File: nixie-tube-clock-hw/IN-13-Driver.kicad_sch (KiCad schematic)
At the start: 7 parts, among them Q50 FZT857TA

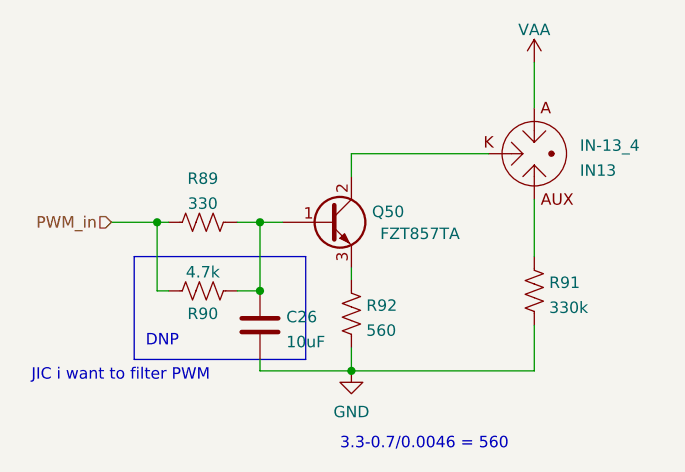
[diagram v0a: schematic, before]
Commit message: fab stuff
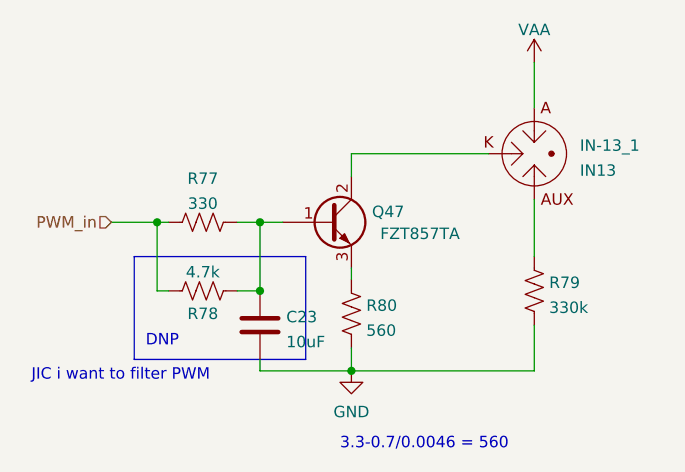
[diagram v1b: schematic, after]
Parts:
- renumbered C26 to C23, IN-13_4 to IN-13_1, Q50 to Q47, R89 to R77, R90 to R78, R91 to R79, R92 to R80
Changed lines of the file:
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@@
   (symbol (lib_id "power:VAA") (at 149.86 68.58 0)
     (in_bom yes) (on_board yes) (fields_autoplaced)
-    (property "Reference" "#PWR0117" (id 0) (at 149.86 72.39 0)
+    (property "Reference" "#PWR0111" (id 0) (at 149.86 72.39 0)
       (effects (font (size 1.27 1.27)) hide)
     )
@@
   (symbol (lib_id "Device:C") (at 119.38 97.79 0)
     (in_bom yes) (on_board yes) (fields_autoplaced)
-    (property "Reference" "C26" (id 0) (at 122.301 96.8815 0)
+    (property "Reference" "C23" (id 0) (at 122.301 96.8815 0)
       (effects (font (size 1.27 1.27)) (justify left))
     )
@@
   (symbol (lib_id "nixie-tube-clock:IN13") (at 149.86 78.74 0)
     (in_bom yes) (on_board yes) (fields_autoplaced)
-    (property "Reference" "IN-13_4" (id 0) (at 154.9287 77.8315 0)
+    (property "Reference" "IN-13_1" (id 0) (at 154.9287 77.8315 0)
       (effects (font (size 1.27 1.27)) (justify left))
     )
@@
   (symbol (lib_id "Device:Q_NPN_BCE") (at 127 86.36 0)
     (in_bom yes) (on_board yes)
-    (property "Reference" "Q50" (id 0) (at 131.826 85.1916 0)
+    (property "Reference" "Q47" (id 0) (at 131.826 85.1916 0)
       (effects (font (size 1.27 1.27)) (justify left))
     )
@@
   (symbol (lib_id "power:GND") (at 129.54 102.87 0)
     (in_bom yes) (on_board yes) (fields_autoplaced)
-    (property "Reference" "#PWR0118" (id 0) (at 129.54 109.22 0)
+    (property "Reference" "#PWR0112" (id 0) (at 129.54 109.22 0)
       (effects (font (size 1.27 1.27)) hide)
     )
@@
   (symbol (lib_id "Device:R_US") (at 149.86 93.98 0)
     (in_bom yes) (on_board yes) (fields_autoplaced)
-    (property "Reference" "R91" (id 0) (at 151.511 93.0715 0)
+    (property "Reference" "R79" (id 0) (at 151.511 93.0715 0)
       (effects (font (size 1.27 1.27)) (justify left))
     )
@@
   (symbol (lib_id "Device:R_US") (at 113.03 93.98 90)
     (in_bom yes) (on_board yes)
-    (property "Reference" "R90" (id 0) (at 113.03 96.52 90))
+    (property "Reference" "R78" (id 0) (at 113.03 96.52 90))
     (property "Value" "4.7k" (id 1) (at 113.03 91.8996 90))
     (property "Footprint" "Resistor_SMD:R_0805_2012Metric" (id 2) (at 113.284 92.964 90)
@@
   (symbol (lib_id "Device:R_US") (at 113.03 86.36 90)
     (in_bom yes) (on_board yes) (fields_autoplaced)
-    (property "Reference" "R89" (id 0) (at 113.03 81.5045 90))
+    (property "Reference" "R77" (id 0) (at 113.03 81.5045 90))
     (property "Value" "330" (id 1) (at 113.03 84.2796 90))
     (property "Footprint" "Resistor_SMD:R_0805_2012Metric" (id 2) (at 113.284 85.344 90)
@@
   (symbol (lib_id "Device:R_US") (at 129.54 96.52 0)
     (in_bom yes) (on_board yes) (fields_autoplaced)
-    (property "Reference" "R92" (id 0) (at 131.191 95.6115 0)
+    (property "Reference" "R80" (id 0) (at 131.191 95.6115 0)
       (effects (font (size 1.27 1.27)) (justify left))
     )

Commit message: minor board / part changes
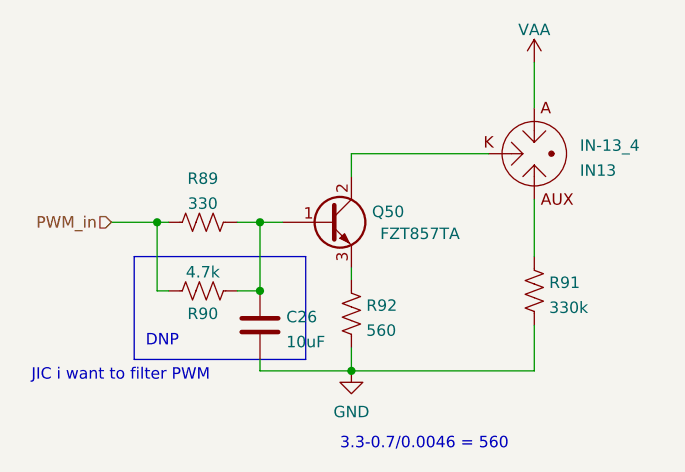
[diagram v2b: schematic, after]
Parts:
- renumbered C23 to C26, IN-13_1 to IN-13_4, Q47 to Q50, R77 to R89, R78 to R90, R79 to R91, R80 to R92
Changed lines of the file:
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@@
   (symbol (lib_id "power:VAA") (at 149.86 68.58 0)
     (in_bom yes) (on_board yes) (fields_autoplaced)
-    (property "Reference" "#PWR0111" (id 0) (at 149.86 72.39 0)
+    (property "Reference" "#PWR0117" (id 0) (at 149.86 72.39 0)
       (effects (font (size 1.27 1.27)) hide)
     )
@@
   (symbol (lib_id "Device:C") (at 119.38 97.79 0)
     (in_bom yes) (on_board yes) (fields_autoplaced)
-    (property "Reference" "C23" (id 0) (at 122.301 96.8815 0)
+    (property "Reference" "C26" (id 0) (at 122.301 96.8815 0)
       (effects (font (size 1.27 1.27)) (justify left))
     )
@@
   (symbol (lib_id "nixie-tube-clock:IN13") (at 149.86 78.74 0)
     (in_bom yes) (on_board yes) (fields_autoplaced)
-    (property "Reference" "IN-13_1" (id 0) (at 154.9287 77.8315 0)
+    (property "Reference" "IN-13_4" (id 0) (at 154.9287 77.8315 0)
       (effects (font (size 1.27 1.27)) (justify left))
     )
@@
   (symbol (lib_id "Device:Q_NPN_BCE") (at 127 86.36 0)
     (in_bom yes) (on_board yes)
-    (property "Reference" "Q47" (id 0) (at 131.826 85.1916 0)
+    (property "Reference" "Q50" (id 0) (at 131.826 85.1916 0)
       (effects (font (size 1.27 1.27)) (justify left))
     )
@@
   (symbol (lib_id "power:GND") (at 129.54 102.87 0)
     (in_bom yes) (on_board yes) (fields_autoplaced)
-    (property "Reference" "#PWR0112" (id 0) (at 129.54 109.22 0)
+    (property "Reference" "#PWR0118" (id 0) (at 129.54 109.22 0)
       (effects (font (size 1.27 1.27)) hide)
     )
@@
   (symbol (lib_id "Device:R_US") (at 149.86 93.98 0)
     (in_bom yes) (on_board yes) (fields_autoplaced)
-    (property "Reference" "R79" (id 0) (at 151.511 93.0715 0)
+    (property "Reference" "R91" (id 0) (at 151.511 93.0715 0)
       (effects (font (size 1.27 1.27)) (justify left))
     )
@@
   (symbol (lib_id "Device:R_US") (at 113.03 93.98 90)
     (in_bom yes) (on_board yes)
-    (property "Reference" "R78" (id 0) (at 113.03 96.52 90))
+    (property "Reference" "R90" (id 0) (at 113.03 96.52 90))
     (property "Value" "4.7k" (id 1) (at 113.03 91.8996 90))
     (property "Footprint" "Resistor_SMD:R_0805_2012Metric" (id 2) (at 113.284 92.964 90)
@@
   (symbol (lib_id "Device:R_US") (at 113.03 86.36 90)
     (in_bom yes) (on_board yes) (fields_autoplaced)
-    (property "Reference" "R77" (id 0) (at 113.03 81.5045 90))
+    (property "Reference" "R89" (id 0) (at 113.03 81.5045 90))
     (property "Value" "330" (id 1) (at 113.03 84.2796 90))
     (property "Footprint" "Resistor_SMD:R_0805_2012Metric" (id 2) (at 113.284 85.344 90)
@@
   (symbol (lib_id "Device:R_US") (at 129.54 96.52 0)
     (in_bom yes) (on_board yes) (fields_autoplaced)
-    (property "Reference" "R80" (id 0) (at 131.191 95.6115 0)
+    (property "Reference" "R92" (id 0) (at 131.191 95.6115 0)
       (effects (font (size 1.27 1.27)) (justify left))
     )

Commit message: 1
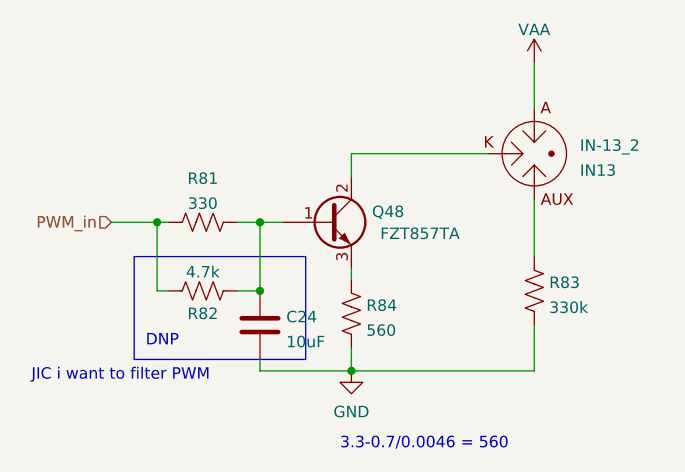
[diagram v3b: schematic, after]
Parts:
- renumbered C26 to C24, IN-13_4 to IN-13_2, Q50 to Q48, R89 to R81, R90 to R82, R91 to R83, R92 to R84
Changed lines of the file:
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@@
   (symbol (lib_id "power:VAA") (at 149.86 68.58 0)
     (in_bom yes) (on_board yes) (fields_autoplaced)
-    (property "Reference" "#PWR0117" (id 0) (at 149.86 72.39 0)
+    (property "Reference" "#PWR0113" (id 0) (at 149.86 72.39 0)
       (effects (font (size 1.27 1.27)) hide)
     )
@@
   (symbol (lib_id "Device:C") (at 119.38 97.79 0)
     (in_bom yes) (on_board yes) (fields_autoplaced)
-    (property "Reference" "C26" (id 0) (at 122.301 96.8815 0)
+    (property "Reference" "C24" (id 0) (at 122.301 96.8815 0)
       (effects (font (size 1.27 1.27)) (justify left))
     )
@@
   (symbol (lib_id "nixie-tube-clock:IN13") (at 149.86 78.74 0)
     (in_bom yes) (on_board yes) (fields_autoplaced)
-    (property "Reference" "IN-13_4" (id 0) (at 154.9287 77.8315 0)
+    (property "Reference" "IN-13_2" (id 0) (at 154.9287 77.8315 0)
       (effects (font (size 1.27 1.27)) (justify left))
     )
@@
   (symbol (lib_id "Device:Q_NPN_BCE") (at 127 86.36 0)
     (in_bom yes) (on_board yes)
-    (property "Reference" "Q50" (id 0) (at 131.826 85.1916 0)
+    (property "Reference" "Q48" (id 0) (at 131.826 85.1916 0)
       (effects (font (size 1.27 1.27)) (justify left))
     )
@@
   (symbol (lib_id "power:GND") (at 129.54 102.87 0)
     (in_bom yes) (on_board yes) (fields_autoplaced)
-    (property "Reference" "#PWR0118" (id 0) (at 129.54 109.22 0)
+    (property "Reference" "#PWR0114" (id 0) (at 129.54 109.22 0)
       (effects (font (size 1.27 1.27)) hide)
     )
@@
   (symbol (lib_id "Device:R_US") (at 149.86 93.98 0)
     (in_bom yes) (on_board yes) (fields_autoplaced)
-    (property "Reference" "R91" (id 0) (at 151.511 93.0715 0)
+    (property "Reference" "R83" (id 0) (at 151.511 93.0715 0)
       (effects (font (size 1.27 1.27)) (justify left))
     )
@@
   (symbol (lib_id "Device:R_US") (at 113.03 93.98 90)
     (in_bom yes) (on_board yes)
-    (property "Reference" "R90" (id 0) (at 113.03 96.52 90))
+    (property "Reference" "R82" (id 0) (at 113.03 96.52 90))
     (property "Value" "4.7k" (id 1) (at 113.03 91.8996 90))
     (property "Footprint" "Resistor_SMD:R_0805_2012Metric" (id 2) (at 113.284 92.964 90)
@@
   (symbol (lib_id "Device:R_US") (at 113.03 86.36 90)
     (in_bom yes) (on_board yes) (fields_autoplaced)
-    (property "Reference" "R89" (id 0) (at 113.03 81.5045 90))
+    (property "Reference" "R81" (id 0) (at 113.03 81.5045 90))
     (property "Value" "330" (id 1) (at 113.03 84.2796 90))
     (property "Footprint" "Resistor_SMD:R_0805_2012Metric" (id 2) (at 113.284 85.344 90)
@@
   (symbol (lib_id "Device:R_US") (at 129.54 96.52 0)
     (in_bom yes) (on_board yes) (fields_autoplaced)
-    (property "Reference" "R92" (id 0) (at 131.191 95.6115 0)
+    (property "Reference" "R84" (id 0) (at 131.191 95.6115 0)
       (effects (font (size 1.27 1.27)) (justify left))
     )

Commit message: 1
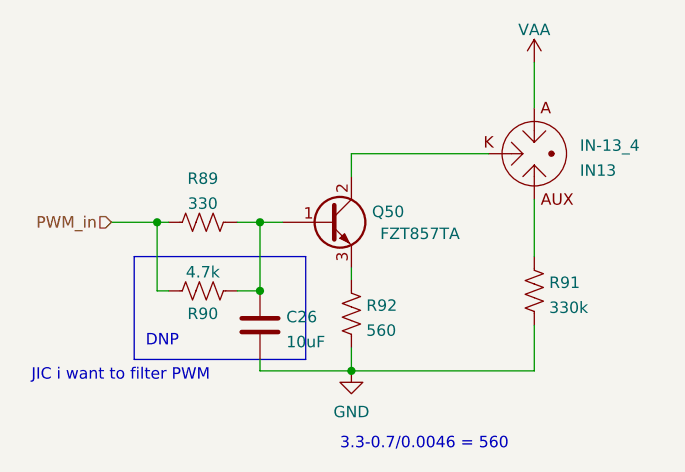
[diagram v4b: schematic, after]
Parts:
- renumbered C24 to C26, IN-13_2 to IN-13_4, Q48 to Q50, R81 to R89, R82 to R90, R83 to R91, R84 to R92
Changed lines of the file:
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@@
   (symbol (lib_id "power:VAA") (at 149.86 68.58 0)
     (in_bom yes) (on_board yes) (fields_autoplaced)
-    (property "Reference" "#PWR0113" (id 0) (at 149.86 72.39 0)
+    (property "Reference" "#PWR0117" (id 0) (at 149.86 72.39 0)
       (effects (font (size 1.27 1.27)) hide)
     )
@@
   (symbol (lib_id "Device:C") (at 119.38 97.79 0)
     (in_bom yes) (on_board yes) (fields_autoplaced)
-    (property "Reference" "C24" (id 0) (at 122.301 96.8815 0)
+    (property "Reference" "C26" (id 0) (at 122.301 96.8815 0)
       (effects (font (size 1.27 1.27)) (justify left))
     )
@@
   (symbol (lib_id "nixie-tube-clock:IN13") (at 149.86 78.74 0)
     (in_bom yes) (on_board yes) (fields_autoplaced)
-    (property "Reference" "IN-13_2" (id 0) (at 154.9287 77.8315 0)
+    (property "Reference" "IN-13_4" (id 0) (at 154.9287 77.8315 0)
       (effects (font (size 1.27 1.27)) (justify left))
     )
@@
   (symbol (lib_id "Device:Q_NPN_BCE") (at 127 86.36 0)
     (in_bom yes) (on_board yes)
-    (property "Reference" "Q48" (id 0) (at 131.826 85.1916 0)
+    (property "Reference" "Q50" (id 0) (at 131.826 85.1916 0)
       (effects (font (size 1.27 1.27)) (justify left))
     )
@@
   (symbol (lib_id "power:GND") (at 129.54 102.87 0)
     (in_bom yes) (on_board yes) (fields_autoplaced)
-    (property "Reference" "#PWR0114" (id 0) (at 129.54 109.22 0)
+    (property "Reference" "#PWR0118" (id 0) (at 129.54 109.22 0)
       (effects (font (size 1.27 1.27)) hide)
     )
@@
   (symbol (lib_id "Device:R_US") (at 149.86 93.98 0)
     (in_bom yes) (on_board yes) (fields_autoplaced)
-    (property "Reference" "R83" (id 0) (at 151.511 93.0715 0)
+    (property "Reference" "R91" (id 0) (at 151.511 93.0715 0)
       (effects (font (size 1.27 1.27)) (justify left))
     )
@@
   (symbol (lib_id "Device:R_US") (at 113.03 93.98 90)
     (in_bom yes) (on_board yes)
-    (property "Reference" "R82" (id 0) (at 113.03 96.52 90))
+    (property "Reference" "R90" (id 0) (at 113.03 96.52 90))
     (property "Value" "4.7k" (id 1) (at 113.03 91.8996 90))
     (property "Footprint" "Resistor_SMD:R_0805_2012Metric" (id 2) (at 113.284 92.964 90)
@@
   (symbol (lib_id "Device:R_US") (at 113.03 86.36 90)
     (in_bom yes) (on_board yes) (fields_autoplaced)
-    (property "Reference" "R81" (id 0) (at 113.03 81.5045 90))
+    (property "Reference" "R89" (id 0) (at 113.03 81.5045 90))
     (property "Value" "330" (id 1) (at 113.03 84.2796 90))
     (property "Footprint" "Resistor_SMD:R_0805_2012Metric" (id 2) (at 113.284 85.344 90)
@@
   (symbol (lib_id "Device:R_US") (at 129.54 96.52 0)
     (in_bom yes) (on_board yes) (fields_autoplaced)
-    (property "Reference" "R84" (id 0) (at 131.191 95.6115 0)
+    (property "Reference" "R92" (id 0) (at 131.191 95.6115 0)
       (effects (font (size 1.27 1.27)) (justify left))
     )
